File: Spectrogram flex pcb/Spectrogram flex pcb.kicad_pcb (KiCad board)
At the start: 2 copper layers, 153.2 x 54.5 mm, 10 parts

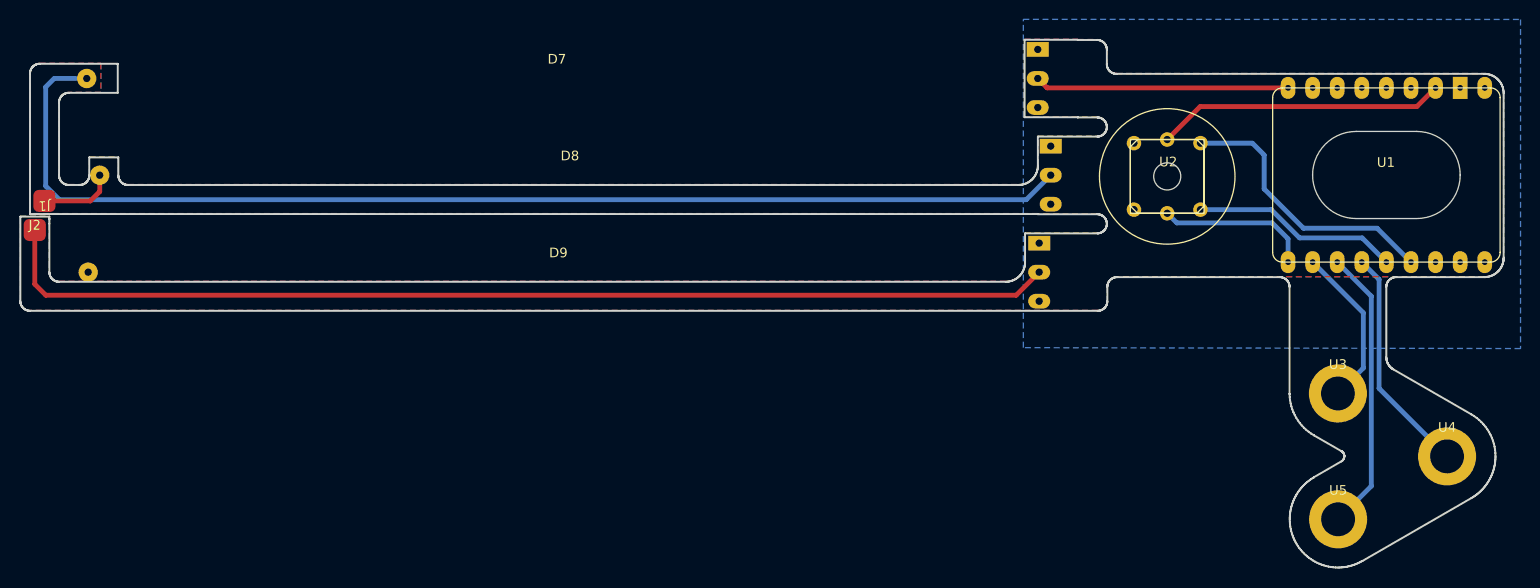
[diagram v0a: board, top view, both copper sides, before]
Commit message: Updating Flex PCB
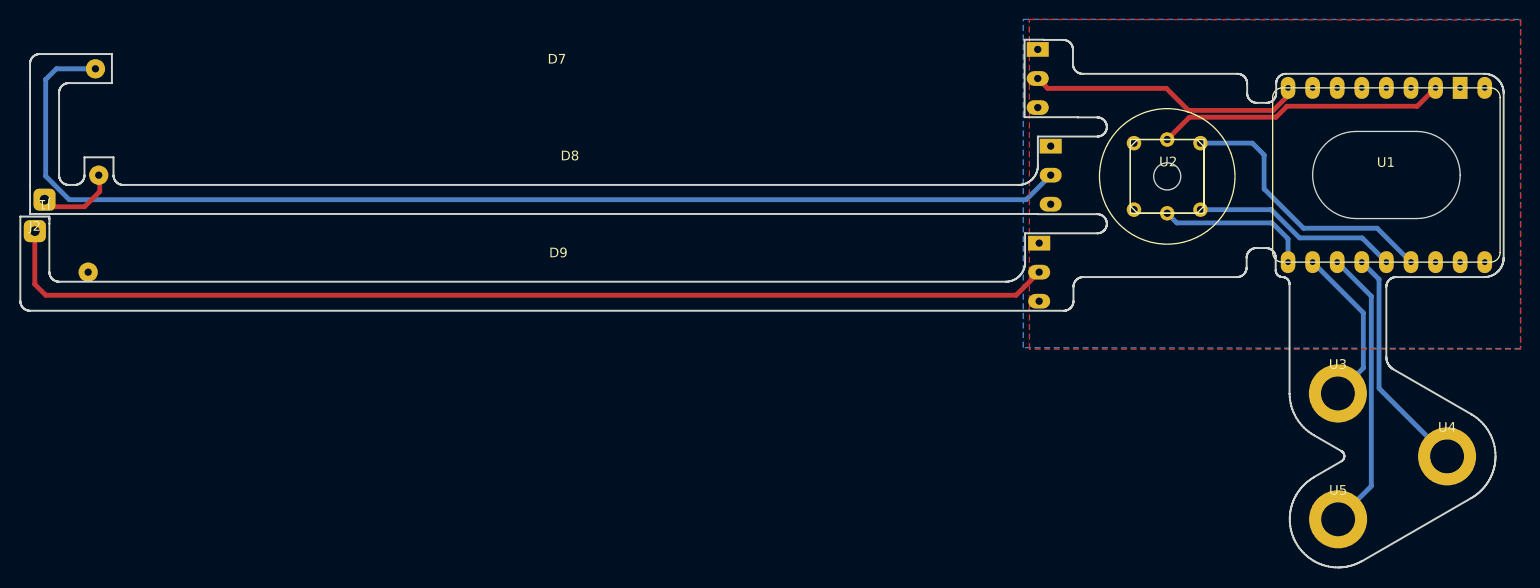
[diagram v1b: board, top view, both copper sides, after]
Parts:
- moved J1 0.13 mm to (81.0, 71.8)
- moved J2 0.12 mm to (80.0, 75.0)
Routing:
- net Net-(D7-Din): track 26.3 -> 28.7 mm
- net Net-(D7-Dout): track 119.2 -> 121.5 mm
- net Net-(D8-Dout): track 7.84 -> 9.04 mm
- removed copper zone on B.Cu, net +5V
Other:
- outline, holes or cut-outs redrawn
